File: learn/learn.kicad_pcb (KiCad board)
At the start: 2 copper layers, 12 parts, among them Q1 PNP, SW1 SW_SPDT

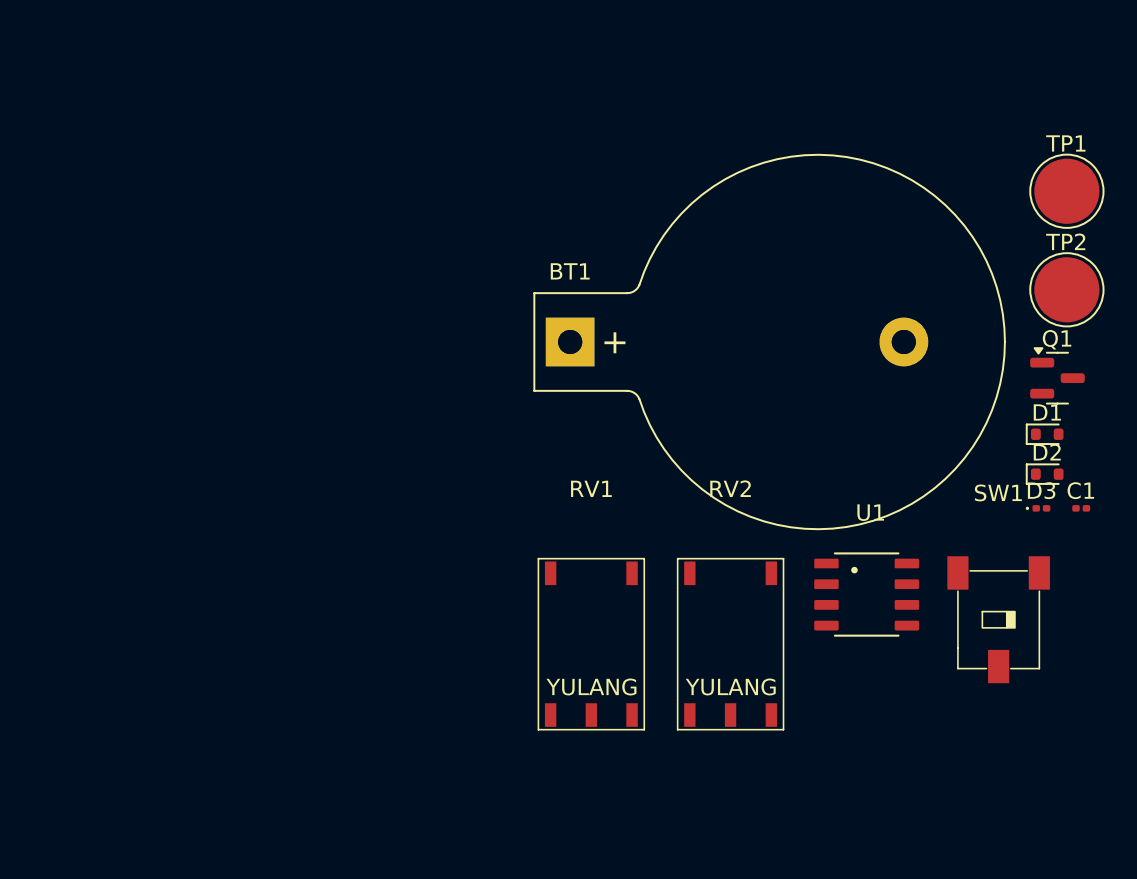
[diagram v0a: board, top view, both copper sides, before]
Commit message: PCB Board Design
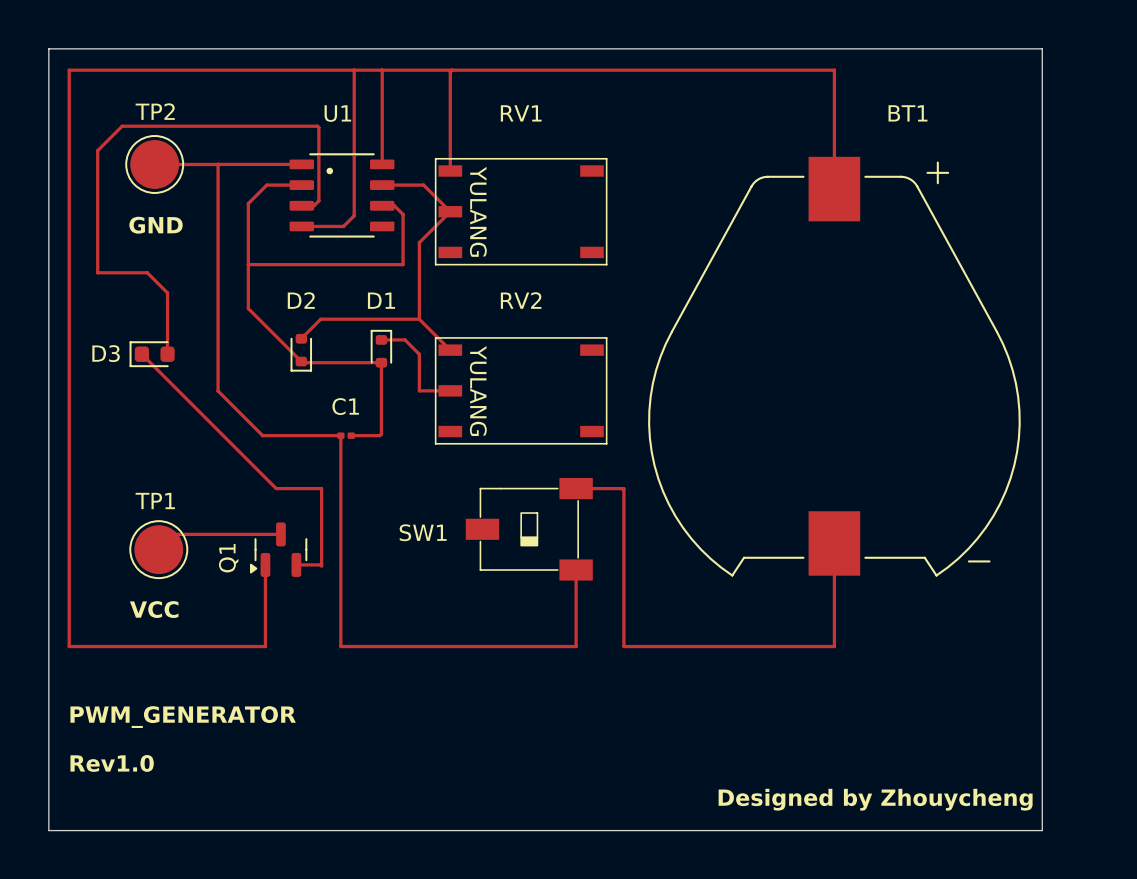
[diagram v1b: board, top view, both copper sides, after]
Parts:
- BT1: value Battery -> 1061; footprint Battery:BatteryHolder_Keystone_103_1x20mm -> Learn:BAT_1061
- D3: footprint LED_SMD:LED_0201_0603Metric -> LED_SMD:LED_0603_1608Metric
- TP1, TP2: footprint TestPoint:TestPoint_Pad_D4.0mm -> TestPoint:TestPoint_Pad_D3.0mm
- moved TP1 59.9 mm to (104.8, 108.8)
- moved TP2 56.5 mm to (104.5, 85.1)
- moved D3 55.3 mm to (104.5, 96.8)
- moved Q1 48.8 mm to (112.2, 108.8), turned to 90 degrees
- moved D2 46.4 mm to (113.5, 96.5), turned to 90 degrees
- moved C1 45.4 mm to (116.2, 101.8), turned to 180 degrees
- moved D1 41.2 mm to (118.4, 96.6), turned to -90 degrees
- moved U1 40.5 mm to (116.0, 87.0)
- moved SW1 29.4 mm to (127.5, 107.5), turned to -90 degrees
- moved RV1 26.9 mm to (127.0, 88.0), turned to -90 degrees
- moved RV2 20.2 mm to (127.0, 99.0), turned to -90 degrees
- moved BT1 16.3 mm to (146.2, 97.5), turned to 180 degrees
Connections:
- net GND renamed Net-(SW1-C)
- Q1 pad 1: Net-(BT1-+) -> Net-(Q1-C)
- RV1 pad 1: Net-(BT1-+) -> Net-(Q1-C)
- SW1 pad 2: Net-(BT1--) -> Net-(SW1-B)
- U1 pad 4: Net-(BT1-+) -> Net-(Q1-C)
- U1 pad 8: Net-(BT1-+) -> Net-(Q1-C)
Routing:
- net Net-(Q1-C): track 0.00 -> 131.2 mm
- net Net-(SW1-C): track 0.00 -> 63.7 mm
- net Net-(D1-A): track 0.00 -> 40.1 mm
- net Net-(D3-A): track 0.00 -> 36.0 mm
- net Net-(SW1-B): track 0.00 -> 31.9 mm
- net Net-(D2-A): track 0.00 -> 22.7 mm
- net Net-(D3-K): track 0.00 -> 20.8 mm
- net Net-(Q1-E): track 0.00 -> 7.89 mm
- net Net-(D1-K): track 0.00 -> 6.84 mm
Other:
- board outline added: 61 x 48 mm
- board text added: "Designed by Zhouycheng"
- board text added: "GND"
- board text added: "PWM_GENERATOR"
- board text added: "Rev1.0"
- board text added: "VCC"

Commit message: fix pcb bugs
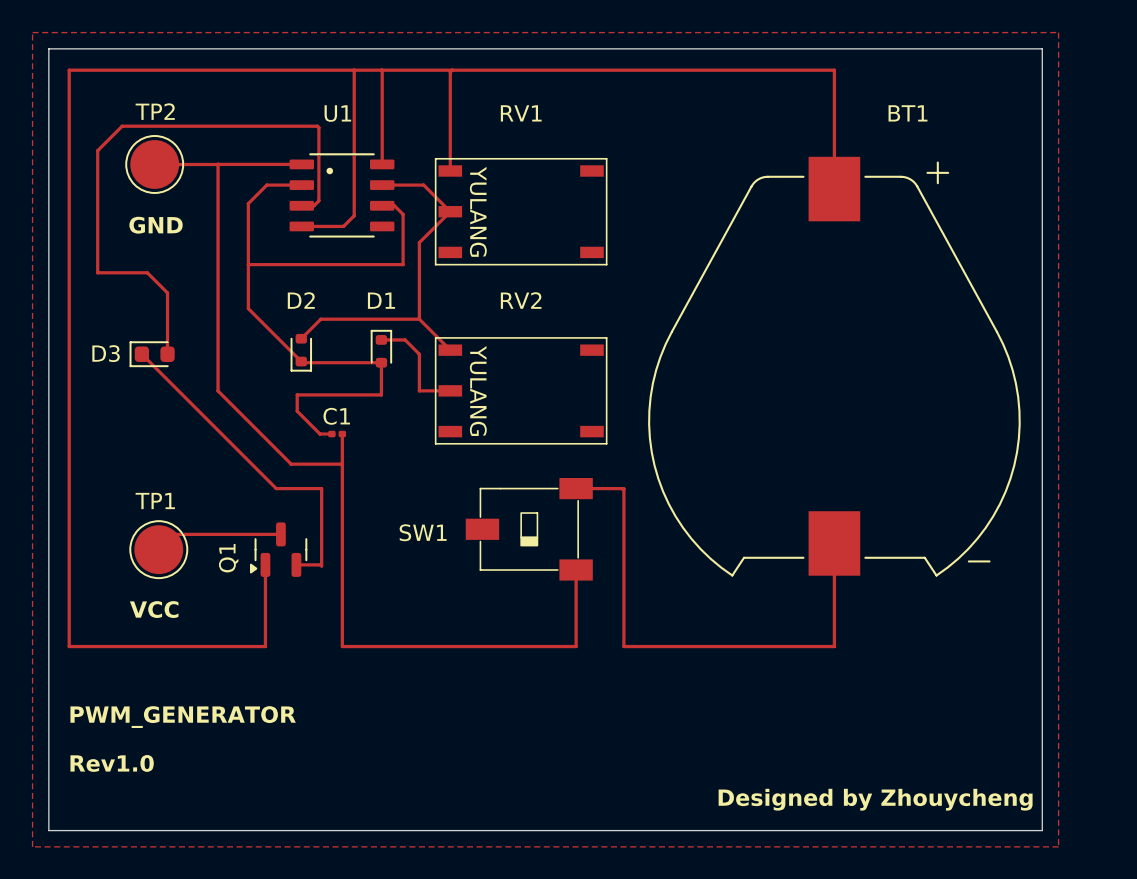
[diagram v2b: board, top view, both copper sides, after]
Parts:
- moved C1 0.56 mm to (115.7, 101.7), turned to 0 degrees
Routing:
- net Net-(D1-A): track 40.1 -> 44.7 mm
- net Net-(SW1-C): track 63.7 -> 64.6 mm
- added copper zone on F.Cu, net (none)
